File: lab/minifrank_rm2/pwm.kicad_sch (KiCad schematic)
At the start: 10 parts

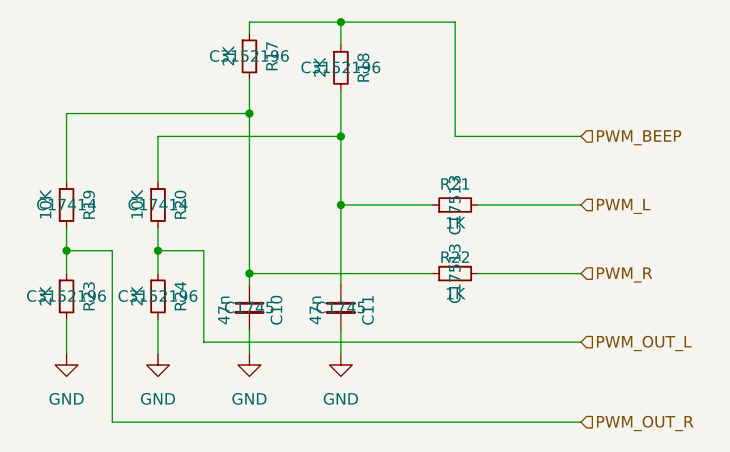
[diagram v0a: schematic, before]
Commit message: MiniFRANK RM2 1.02
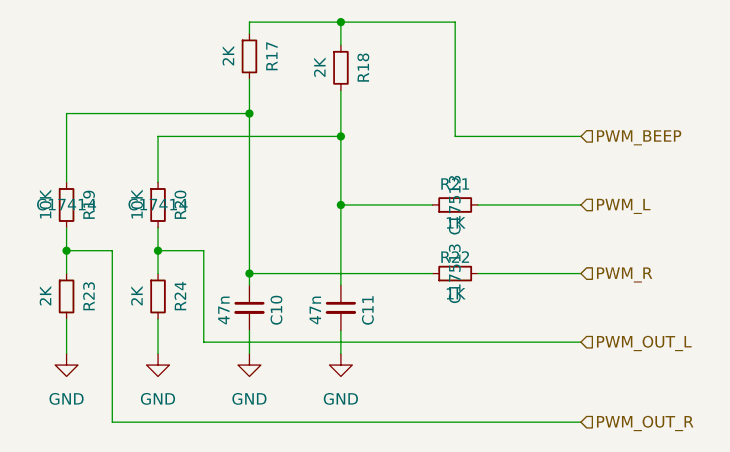
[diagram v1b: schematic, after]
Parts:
- C10, C11: LCSC C1745 -> (none)
- R17, R18, R23, R24: LCSC C3152196 -> (none)
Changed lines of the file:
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@@
 			)
 		)
-		(property "LCSC" "C3152196"
+		(property "LCSC" ""
 			(at 144.78 78.74 0)
 			(effects
@@
 			)
 		)
-		(property "LCSC" "C3152196"
+		(property "LCSC" ""
 			(at 134.62 77.47 0)
 			(effects
@@
 			)
 		)
-		(property "LCSC" "C1745"
+		(property "LCSC" ""
 			(at 134.62 105.41 0)
 			(effects
@@
 			)
 		)
-		(property "LCSC" "C3152196"
+		(property "LCSC" ""
 			(at 124.46 104.14 0)
 			(effects
@@
 			)
 		)
-		(property "LCSC" "C3152196"
+		(property "LCSC" ""
 			(at 114.3 104.14 0)
 			(effects
@@
 			)
 		)
-		(property "LCSC" "C1745"
+		(property "LCSC" ""
 			(at 144.78 105.41 0)
 			(effects
